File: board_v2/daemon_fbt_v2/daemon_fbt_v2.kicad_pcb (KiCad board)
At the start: 2 copper layers, 60 parts, among them IC1 NPM1100-QDAA-R7, IC2 nRF52840-QFAA-F-R7, IC3 MX25U2035FZUI-TR, J1 P70-5100045, J2 P70-5100045, J3 150mAh, Q1 FDV303N, U1 BMM350, U2 BHI360, Y1 ECS-320-8-37B2-CTN-TR

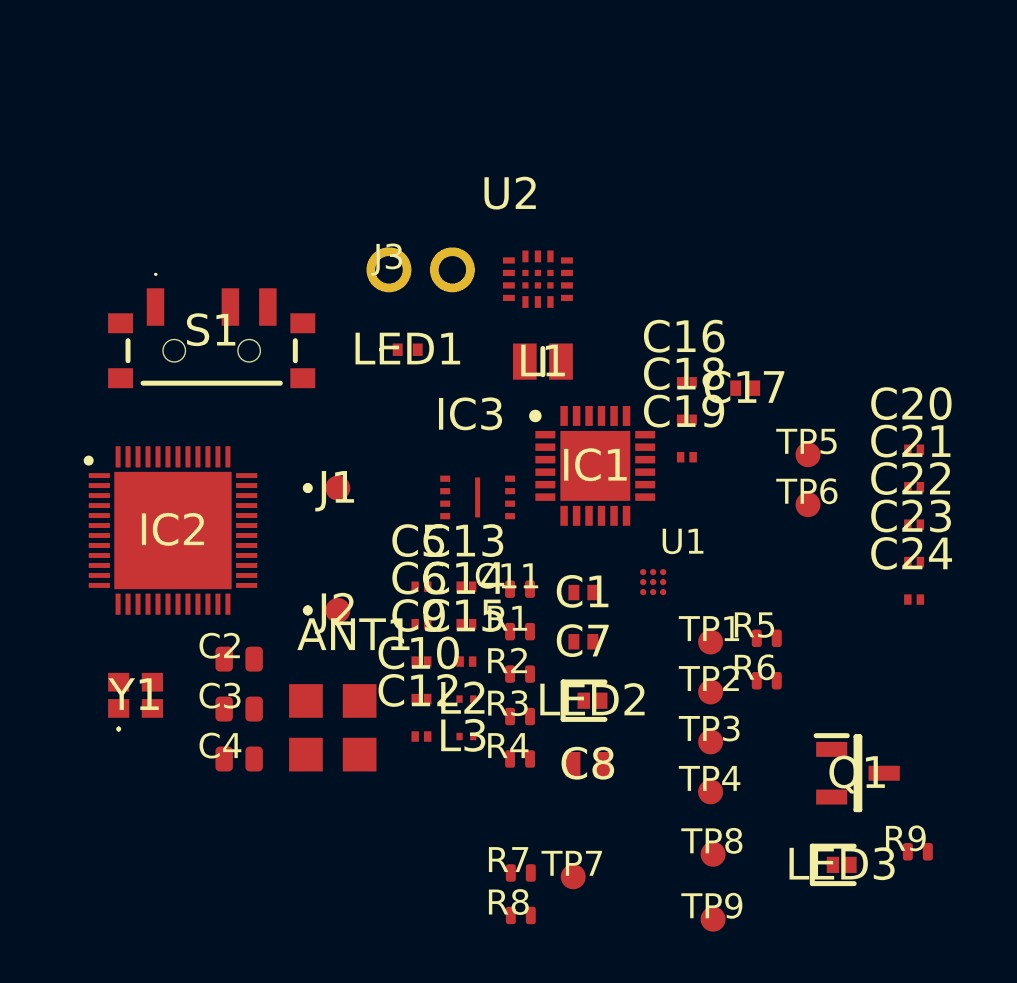
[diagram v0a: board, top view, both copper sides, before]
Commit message: finished redesign; lets hope jlcpcb doesn't kill me
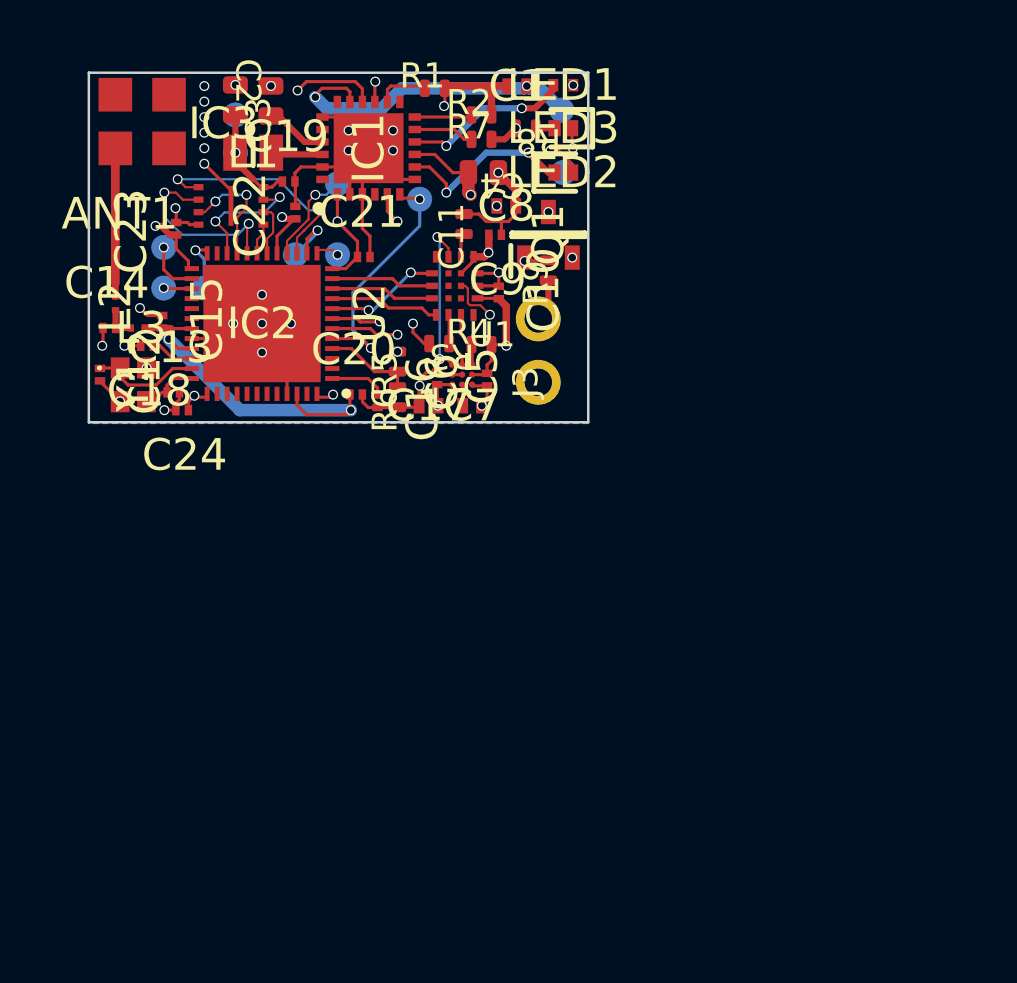
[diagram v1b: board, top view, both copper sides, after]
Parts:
- removed S1: SSSS811101, the_backrooms:SSSS811101
- C8: footprint the_backrooms:CAPC1608X90N -> the_backrooms:CAPC1005X55N
- J1, J2, TP1, TP2, TP3, TP4, TP5, TP6, TP7, TP8, TP9: moved to B.Cu
- moved TP4 33.1 mm to (29.9, 17.7), turned to 180 degrees
- moved TP9 32.5 mm to (28.6, 24.6), turned to 90 degrees
- moved C23 32.4 mm to (27.5, 22.2), turned to 90 degrees
- moved R8 31.5 mm to (42.0, 18.2), turned to 180 degrees
- moved LED3 31.5 mm to (43.0, 18.2), turned to 180 degrees
- moved TP8 30.8 mm to (34.0, 20.4), turned to 90 degrees
- moved TP3 30.3 mm to (29.9, 19.2), turned to 180 degrees
- moved C24 30.3 mm to (27.7, 29.5), turned to 180 degrees
- moved R7 29.4 mm to (39.2, 18.7)
- moved TP7 27.8 mm to (37.2, 21.1), turned to -90 degrees
- moved C22 27.8 mm to (32.3, 21.6), turned to 90 degrees
- moved TP2 27.2 mm to (27.0, 24.6), turned to 180 degrees
- moved TP1 27.0 mm to (27.0, 23.0), turned to 180 degrees
- moved R9 26.9 mm to (42.4, 24.4), turned to 90 degrees
- moved C4 26.1 mm to (40.6, 20.0), turned to 180 degrees
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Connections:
- C8 pad 1: GND -> +1V8
- C8 pad 2: +1V8 -> GND
- J3 pad 1: /VBATTERY -> /VBAT
- R5 pad 2: /VBATTERY -> /VBAT
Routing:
- net GND: track 0.00 -> 51.1 mm, vias 0 -> 30
- net +1V8: track 0.00 -> 33.8 mm, vias 0 -> 11
- net /VBAT: track 0.00 -> 22.0 mm, vias 0 -> 2
- net /DEC_4_6: track 0.00 -> 12.9 mm, vias 0 -> 2
- net VBUS: track 0.00 -> 12.7 mm, vias 0 -> 2
- net /BAT_LOW: track 0.00 -> 10.7 mm, vias 0 -> 2
- net /VSYS: track 0.00 -> 10.2 mm, vias 0 -> 6
- net /SHPACT: track 0.00 -> 9.73 mm, vias 0 -> 2
- net /QSPI_~{CS}: track 0.00 -> 9.14 mm, vias 0 -> 2
- net /BHI360_INT: track 0.00 -> 8.47 mm, vias 0 -> 2
- net /QSPI_1: track 0.00 -> 7.40 mm, vias 0 -> 2
- net /CHG_LED: track 0.00 -> 7.07 mm, vias 0 -> 2
- net /ERR_LED: track 0.00 -> 6.59 mm, vias 0 -> 2
- net /BMM350_INT: track 0.00 -> 6.50 mm, vias 0 -> 2
- net Net-(ANT1-FEED): track 0.00 -> 5.93 mm
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- added copper zone on In2.Cu, net +1V8
- added copper zone on In2.Cu, net /VSYS
- added copper zone on B.Cu, net GND
- added copper zone on In1.Cu, net GND
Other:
- board outline added: 20 x 14 mm
- copper layers 2 -> 4
